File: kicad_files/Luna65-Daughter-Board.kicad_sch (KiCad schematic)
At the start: 34 parts, among them J1 TYPE-C-31-M12_13, J2 Molex Power, J3 JSTPH, U1 MCP73831, U2 USBLC6-2SC6, U3 AP2112, U4 TPS61202DRC

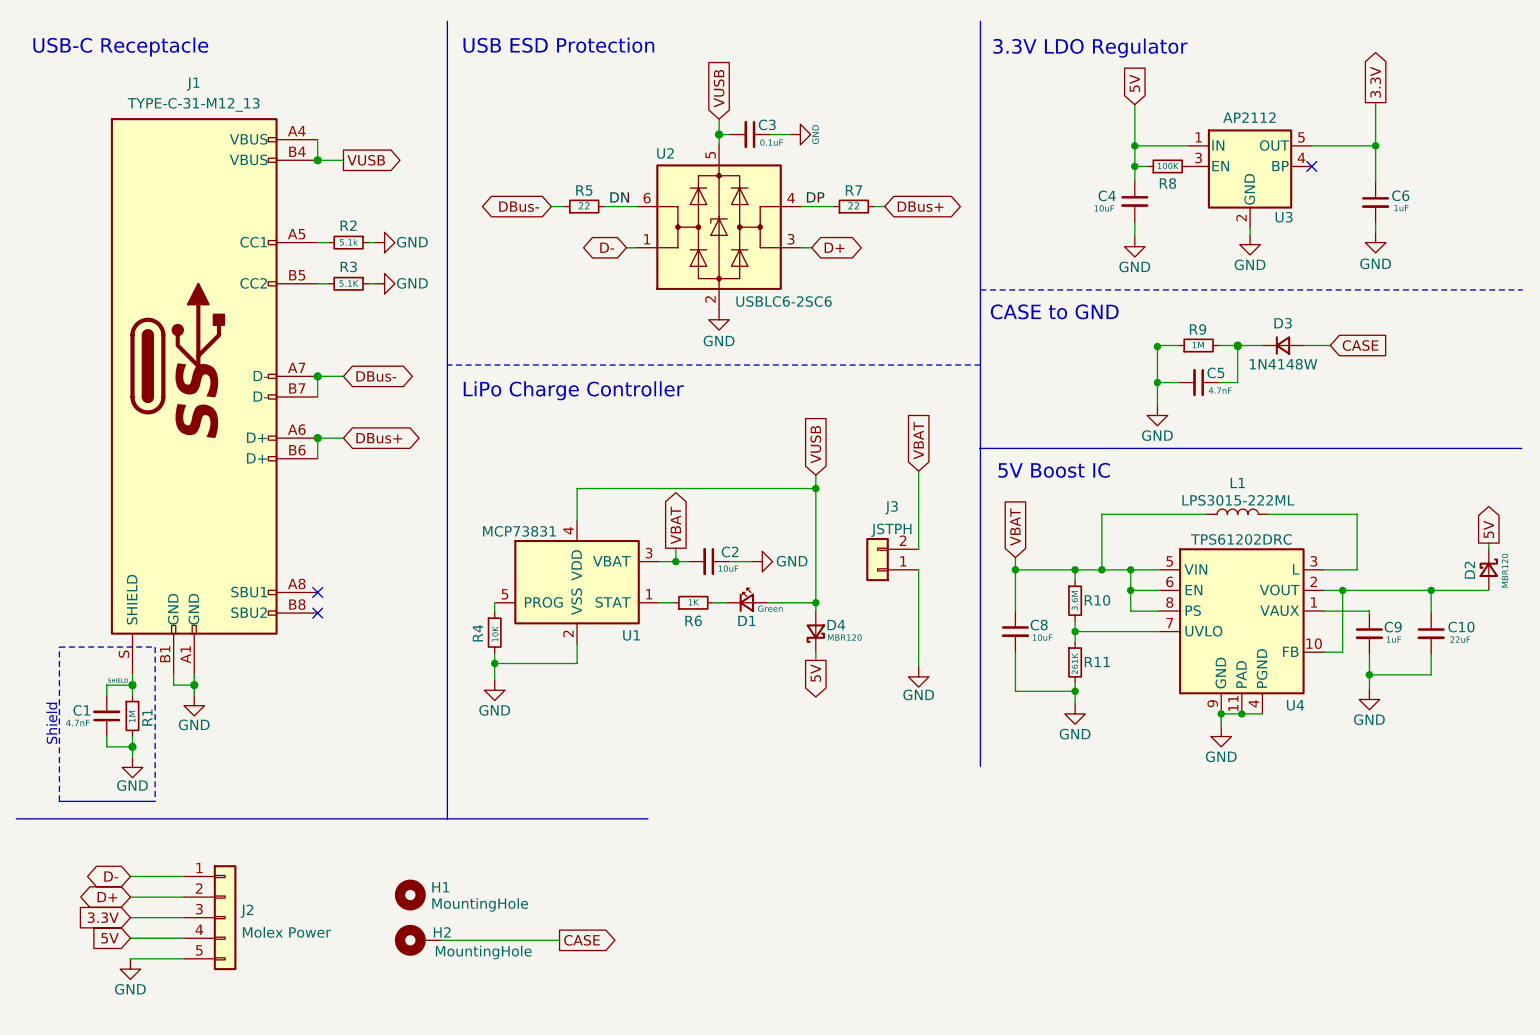
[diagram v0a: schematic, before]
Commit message: DB Rev C
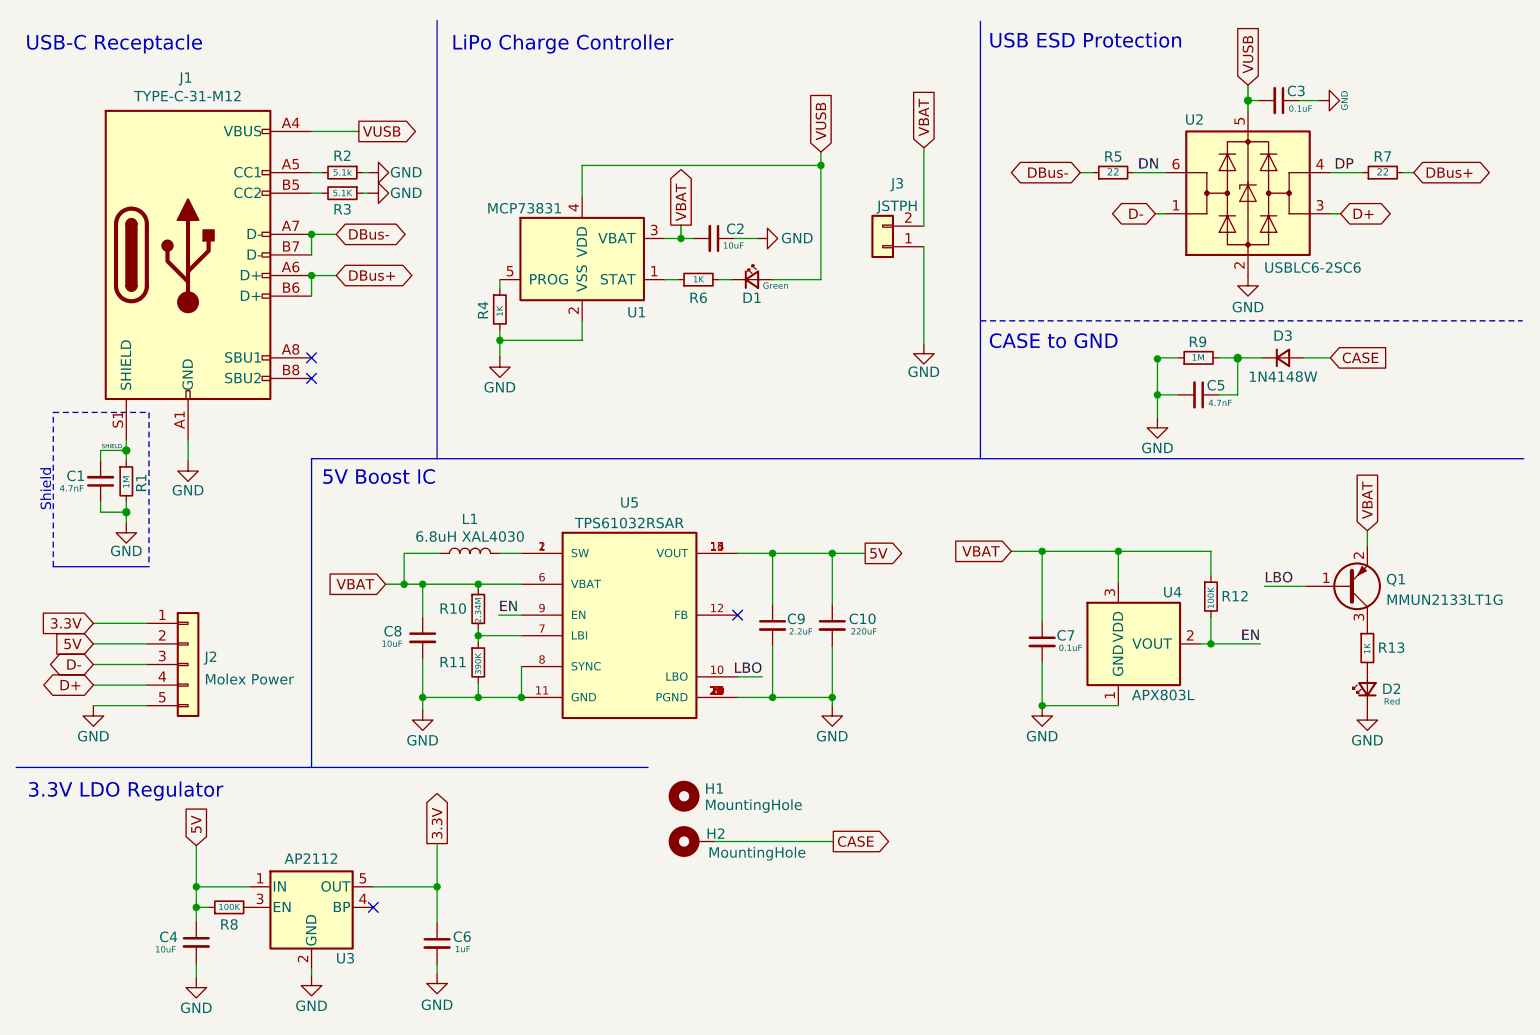
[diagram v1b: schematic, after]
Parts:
- removed D2, D4: MBR120, acheron_Components:D_SOD-123, symbol Device:D_Schottky_Small
- removed U4: TPS61202DRC, Package_SON:Texas_S-PVSON-N10_ThermalVias, symbol Regulator_Switching:TPS61202DRC
- added C7: 0.1uF, acheron_Components:C_0805_2012Metric, symbol Device:C_Small
- added D2: Red, LED_SMD:LED_1206_3216Metric_Pad1.42x1.75mm_HandSolder, symbol Device:LED_Small
- added Q1: MMUN2133LT1G, Package_TO_SOT_SMD:SOT-23, symbol Transistor_BJT:MMBTA92
- added R12: 100K, Resistor_SMD:R_0805_2012Metric, symbol Device:R_Small
- added R13: 1K, Resistor_SMD:R_0805_2012Metric, symbol Device:R_Small
- added U4: APX803L, Package_TO_SOT_SMD:SOT-23, symbol Power_Management:BD49KxxG
- added U5: TPS61032RSAR, Package_DFN_QFN:Texas_S-PVQFN-N16_EP2.7x2.7mm_ThermalVias, symbol TPS61030PWP:TPS61030PWP
- C10: value 22uF -> 220uF; footprint acheron_Components:C_0805_2012Metric -> Capacitor_SMD:C_1206_3216Metric
- C9: value 1uF -> 2.2uF
- J1: value TYPE-C-31-M12_13 -> TYPE-C-31-M12; symbol acheronSymbols:TYPE-C-31-M12_13 -> acheron_Symbols:TYPE-C-31-M-12
- L1: value LPS3015-222ML -> 6.8uH XAL4030; footprint Luna65:LPS3015 -> Luna65:XAL4030
- R10: value 3.6M -> 2.34M
- R11: value 261K -> 390K
- R4: value 10K -> 1K
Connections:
- net 3.3V: now also J2.1 (Pin_1); no longer J2.3 (Pin_3)
- net 5V: now also C10.1, C9.1, J2.2 (Pin_2), U5.13 (VOUT), U5.14 (VOUT), U5.15 (VOUT); no longer J2.4 (Pin_4)
- net D+: now also J2.4 (Pin_4); no longer J2.2 (Pin_2)
- net D-: now also J2.3 (Pin_3); no longer J2.1 (Pin_1)
- net GND: now also C7.2, D2.1 (K), U4.1 (GND), U5.11 (GND), U5.17 (PGND), U5.18 (PGND), U5.19 (PGND), U5.20 (PGND), U5.21 (PGND), U5.22 (PGND), U5.23 (PGND), U5.24 (PGND), U5.25 (PGND), U5.26 (PGND), U5.27 (PGND), U5.28 (PGND), U5.29 (PGND), U5.3 (PGND), U5.4 (PGND), U5.5 (PGND), U5.8 (SYNC)
- net SHIELD: now also J1.S1 (SHIELD); no longer J1.S (SHIELD)
- net VBAT: now also C7.1, Q1.2 (E), R12.1, U4.3 (VDD), U5.6 (VBAT)
- net at R10.2, R11.1: now also U5.7 (LBI)
- net at L1.2: now also U5.1 (SW), U5.2 (SW)
- new net: Q1.3 (C), R13.1
- new net: D2.2 (A), R13.2
- new net EN: R12.2, U4.2 (VOUT), U5.9 (EN)
- new net LBO: Q1.1 (B), U5.10 (LBO)
- no-connect marks 3 -> 4
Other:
- moved on the sheet: C1, C2, C3, C4, C5, C6, D1, D3, H1, H2, J2, J3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
